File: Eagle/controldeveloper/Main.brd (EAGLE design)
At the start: 64 x 81 mm, 21 parts

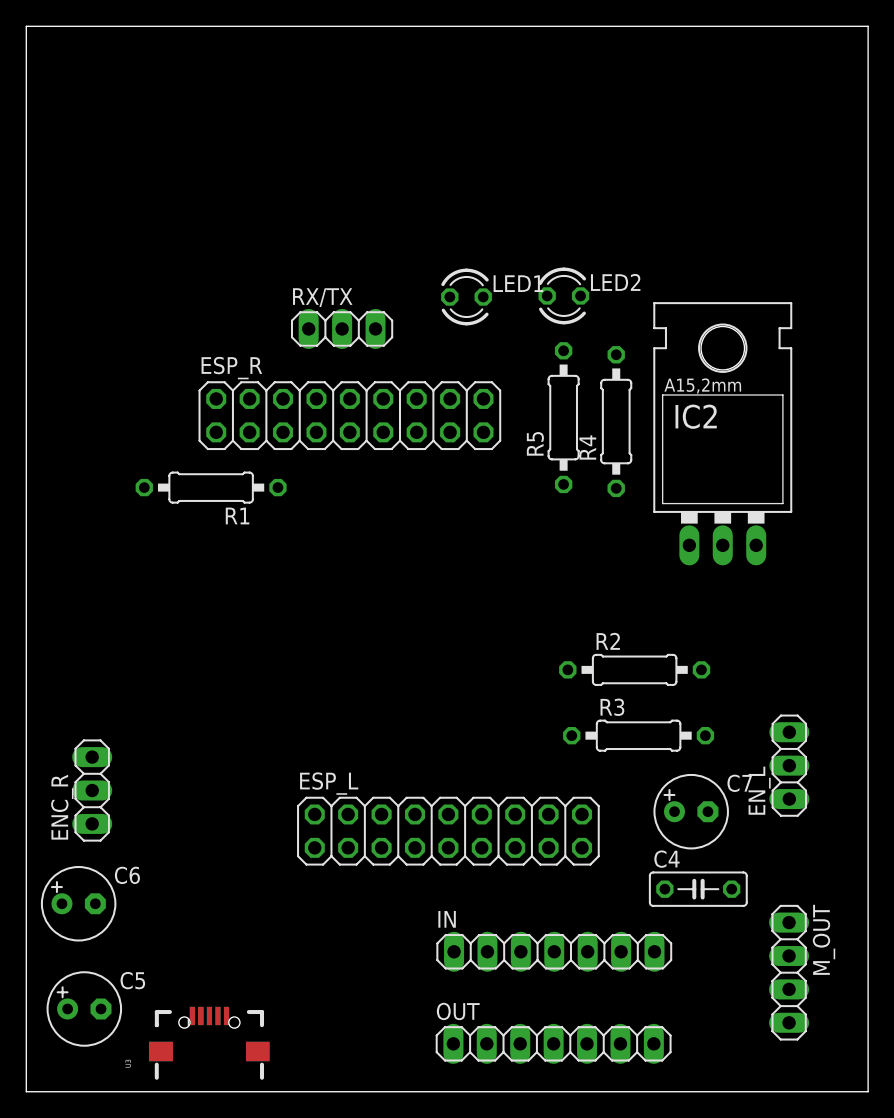
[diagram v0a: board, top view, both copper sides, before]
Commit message: Finished eagle board!
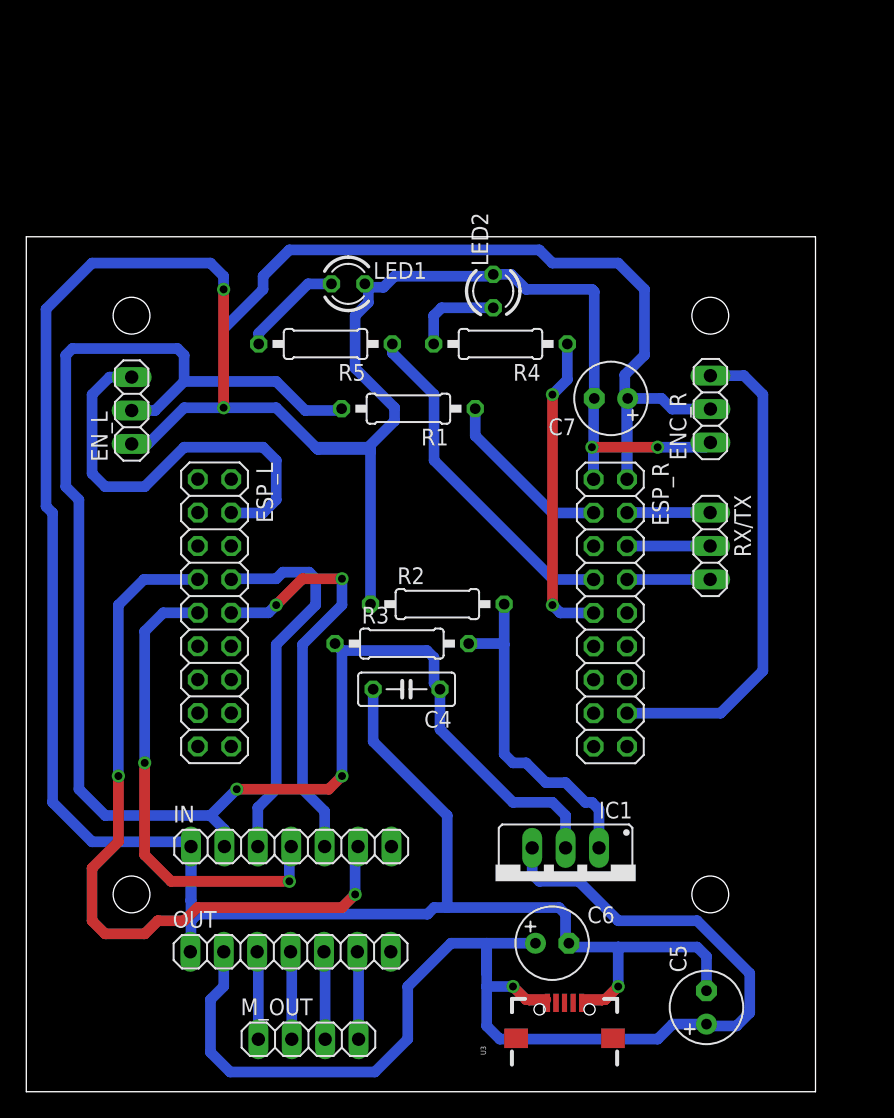
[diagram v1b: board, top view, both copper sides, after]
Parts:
- removed IC2: (no value), v-reg:317TL
- added IC1: (no value), v-reg:317TS
- moved EN_L 56.8 mm to (8.01, 51.8)
- moved ENC_R 55.2 mm to (52.0, 51.9)
- moved C5 47.3 mm to (51.7, 6.41), turned to 90 degrees
- moved M_OUT 36.9 mm to (21.4, 3.99), turned to 0 degrees
- moved C6 36.1 mm to (40.0, 11.3)
- moved RX/TX 32.5 mm to (52.0, 41.5), turned to 270 degrees
- moved C7 32.0 mm to (44.5, 52.7), turned to 180 degrees
- moved U3 27.0 mm to (40.9, 4.06)
- moved C4 26.9 mm to (28.9, 30.6), turned to 180 degrees
- moved ESP_R 24.8 mm to (44.4, 36.4), turned to 270 degrees
- moved ESP_L 24.3 mm to (14.3, 36.4), turned to 270 degrees
- moved IN 21.5 mm to (20.1, 18.6)
- moved OUT 21.2 mm to (20.1, 10.6)
- moved R3 19.3 mm to (28.6, 34.1)
- moved R5 18.9 mm to (22.8, 56.9), turned to 180 degrees
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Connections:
- removed net N$14: ESP_R.8, RX/TX.2
- removed net N$9: ESP_R.10, RX/TX.3
- new net N$5: ESP_R.4, RX/TX.1
- new net N$8: ESP_R.8, RX/TX.3
- net ENC_R: now also ESP_R.16; no longer ESP_R.18
- net GND: now also ESP_R.1; no longer ESP_R.3
- net LED1: now also ESP_R.7; no longer ESP_R.9
- net LED2: now also ESP_R.9; no longer ESP_R.11
- net N$12: now also ESP_R.3; no longer ESP_R.5
- net N$6: now also RX/TX.2; no longer RX/TX.1
- net N$7: now also IC1.1; no longer IC2.1
- net VCC: now also ESP_R.2, IC1.2; no longer ESP_R.4, IC2.2
- net VDD: now also IC1.3; no longer IC2.3
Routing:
- net GND: track 0.00 -> 254.5 mm, vias 0 -> 5
- net VCC: track 0.00 -> 193.7 mm, vias 0 -> 2
- net VDD: track 0.00 -> 100.7 mm, vias 0 -> 1
- net PH2: track 0.00 -> 57.1 mm, vias 0 -> 2
- net ENC_R: track 0.00 -> 37.3 mm
- net PH1: track 0.00 -> 36.2 mm, vias 0 -> 2
- net ENC_L: track 0.00 -> 32.5 mm
- net EN2: track 0.00 -> 31.8 mm, vias 0 -> 2
- net EN1: track 0.00 -> 29.0 mm
- net LED1: track 0.00 -> 26.0 mm
- net N$7: track 0.00 -> 26.0 mm
- net LED2: track 0.00 -> 23.7 mm, vias 0 -> 2
- net N$12: track 0.00 -> 13.5 mm
- net N$13: track 0.00 -> 7.90 mm
- net N$10: track 0.00 -> 6.93 mm
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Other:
- board size 64 x 81 mm -> 60 x 65 mm
